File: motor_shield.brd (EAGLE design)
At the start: 98 x 59.3 mm, 10 parts, among them J1 22-27-2041-04

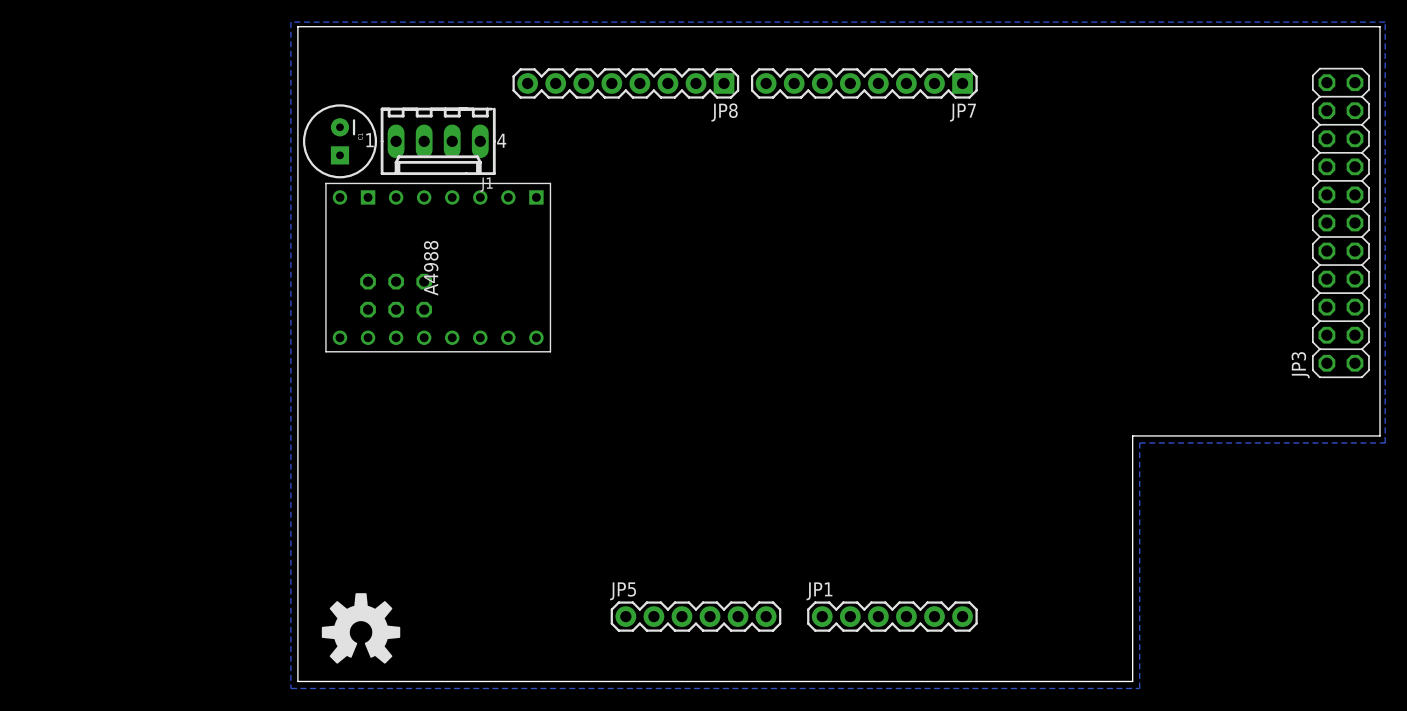
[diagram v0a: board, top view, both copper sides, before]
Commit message: add A4988
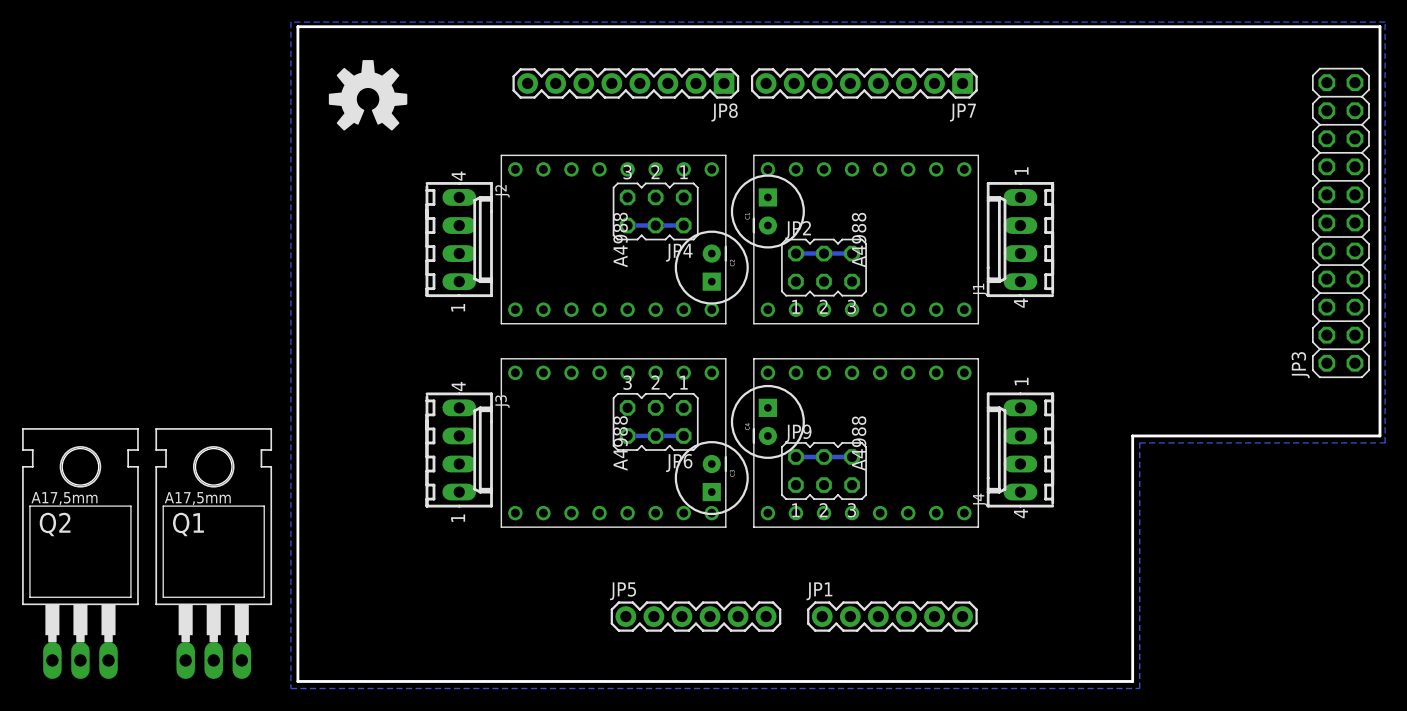
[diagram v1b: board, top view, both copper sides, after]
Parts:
- added C2, C3, C4: (no value), SparkFun:CPOL-RADIAL-100UF-25V
- added J2, J3, J4: 22-27-2041-04, con-molex:6410-04
- added JP4, JP6, JP9: (no value), jumper:JP3Q
- added Q1, Q2: IRLZ44Z, transistor-power:TO220BH
- added U$2, U$3, U$4: A4988, A4988:A4988
- U$1: value (none) -> A4988
- moved J1 53.4 mm to (65.4, 40.0), turned to 90 degrees
- moved OPENHARDWARE 48.3 mm to (6.35, 52.7)
- moved C1 39.3 mm to (42.5, 42.5), turned to 90 degrees
- moved JP2 38.8 mm to (47.6, 37.5), flipped to the top, turned to 0 degrees
- moved U$1 38.8 mm to (51.4, 40.0)
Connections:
- new net N$10: J2.2, U$2.1A
- new net N$11: J2.1, U$2.1B
- new net N$12: JP6.1, U$3.MS1
- new net N$13: JP6.3, U$3.MS2
- new net N$14: JP6.5, U$3.MS3
- new net N$15: J3.4, U$3.2B
- new net N$16: J3.3, U$3.2A
- new net N$17: J3.2, U$3.1A
- new net N$18: J3.1, U$3.1B
- new net N$20: JP9.5, U$4.MS3
- new net N$21: JP9.3, U$4.MS2
- new net N$22: J4.4, U$4.2B
- new net N$23: J4.3, U$4.2A
- new net N$24: J4.2, U$4.1A
- new net N$25: J4.1, U$4.1B
- new net N$26: JP9.1, U$4.MS1
- new net N$27: JP4.1, U$2.MS1
- new net N$28: JP4.3, U$2.MS2
- new net N$29: JP4.5, U$2.MS3
- new net N$8: J2.4, U$2.2B
- new net N$9: J2.3, U$2.2A
- net +24V: now also C2.1, C3.1, C4.1, U$2.VMOT, U$3.VMOT, U$4.VMOT
- net +5V: now also JP2.2, JP2.4, JP2.6, JP4.2, JP4.4, JP4.6, JP6.2, JP6.4, JP6.6, JP9.2, JP9.4, JP9.6, U$2.RESET, U$2.SLEEP, U$2.VDD, U$3.RESET, U$3.SLEEP, U$3.VDD, U$4.RESET, U$4.SLEEP, U$4.VDD; no longer JP2.1, JP2.3, JP2.5
- net GND: now also C2.2, C3.2, C4.2, Q1.S, Q2.S, U$1.GMOT, U$1.GND, U$2.GMOT, U$2.GND, U$3.GMOT, U$3.GND, U$4.GMOT, U$4.GND; no longer U$1.GND1, U$1.GND2
- net N$1: now also J1.4; no longer J1.1
- net N$2: now also J1.3; no longer J1.2
- net N$3: now also J1.2; no longer J1.3
- net N$4: now also J1.1; no longer J1.4
- net N$5: now also JP2.1; no longer JP2.2
- net N$6: now also JP2.3; no longer JP2.4
- net N$7: now also JP2.5; no longer JP2.6
- net P026: now also U$4.ENABLE
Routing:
- net +5V: track 0.00 -> 20.3 mm
